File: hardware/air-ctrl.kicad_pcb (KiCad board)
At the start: 2 copper layers, 35 x 35 mm, 71 parts, among them J1 USB_C_Receptacle_USB2.0_16P, J2 SFV24R-2STE1HLF, J3 Conn_ARM_SWD_TagConnect_TC203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, J4 Conn_01x02, Q1 BSS138, SW1 SW_RST, U1 nRF52832-QFxx, U2 BME688, U3 MCP73871-2CC, U4 MCP1700x-330xxTT, Y1 32MHz, Y2 32.768kHz

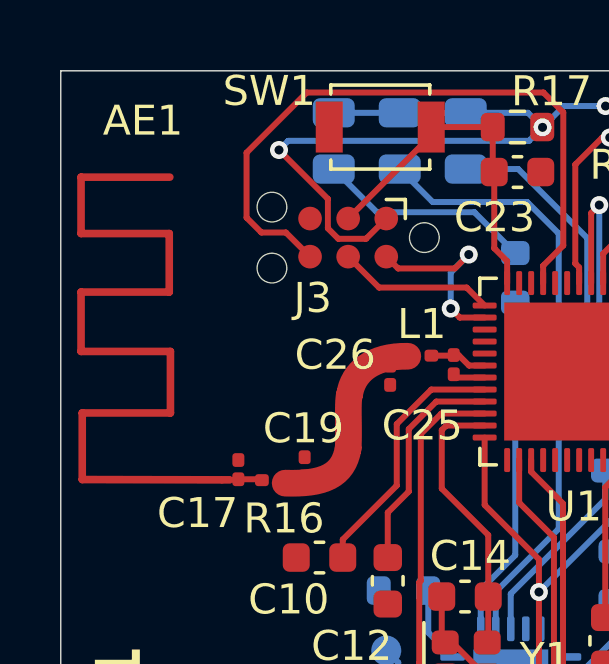
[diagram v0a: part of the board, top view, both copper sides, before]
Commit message: Fixed DRC issues on antenna pad and trace
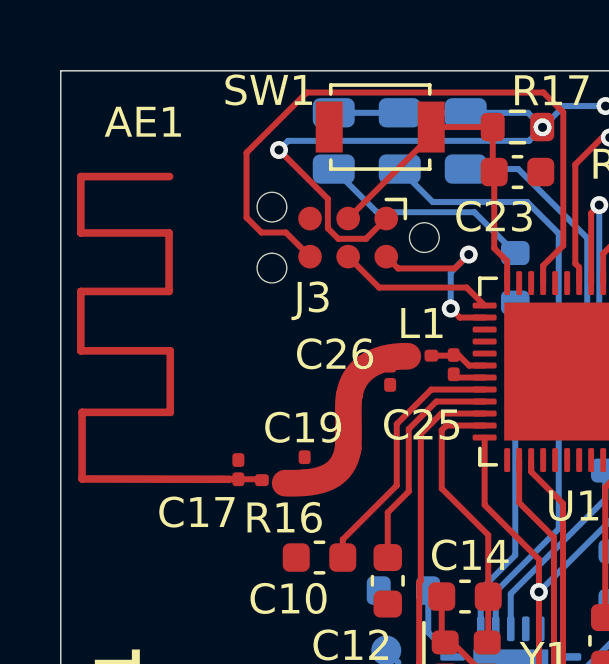
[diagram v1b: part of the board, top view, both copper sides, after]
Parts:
- moved AE1 0.09 mm to (153.7, 48.9)
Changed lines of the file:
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@@
 	(footprint "RF_Antenna:Antenna_BLE"
 		(layer "F.Cu")
-		(at 153.6565 48.81 90)
+		(at 153.71 48.88 90)
 		(property "Reference" "AE1"
 			(at 7.17 -0.9165 0)
@@
 		(net_tie_pad_groups "1")
 		(fp_line
-			(start 5.29 -2.98)
-			(end 5.29 -0.02)
+			(start 5.380104 -3.04)
+			(end 5.380104 -0.08)
 			(stroke
 				(width 0.254)
@@
 		)
 		(fp_line
-			(start 3.41 -2.98)
-			(end 5.29 -2.98)
+			(start 3.500104 -3.04)
+			(end 5.380104 -3.04)
 			(stroke
 				(width 0.254)
@@
 		)
 		(fp_line
-			(start 1.46 -2.98)
-			(end 1.46 -0.04)
+			(start 1.550104 -3.04)
+			(end 1.550104 -0.1)
 			(stroke
 				(width 0.254)
@@
 		)
 		(fp_line
-			(start -0.52 -2.98)
-			(end 1.46 -2.98)
+			(start -0.429896 -3.04)
+			(end 1.550104 -3.04)
 			(stroke
 				(width 0.254)
@@
 		)
 		(fp_line
-			(start -2.57 -2.94)
-			(end -2.57 0)
+			(start -2.479896 -3)
+			(end -2.479896 -0.06)
 			(stroke
 				(width 0.254)
@@
 		)
 		(fp_line
-			(start -4.79 -2.94)
-			(end -2.57 -2.94)
+			(start -4.699896 -3)
+			(end -2.479896 -3)
 			(stroke
 				(width 0.254)
@@
 		)
 		(fp_line
-			(start 3.41 -0.04)
-			(end 3.41 -2.98)
+			(start 3.500104 -0.1)
+			(end 3.500104 -3.04)
 			(stroke
 				(width 0.254)
@@
 		)
 		(fp_line
-			(start 1.46 -0.04)
-			(end 3.41 -0.04)
+			(start 1.550104 -0.1)
+			(end 3.500104 -0.1)
 			(stroke
 				(width 0.254)
@@
 		)
 		(fp_line
-			(start -0.52 0)
-			(end -0.52 -2.98)
+			(start -0.429896 -0.06)
+			(end -0.429896 -3.04)
 			(stroke
 				(width 0.254)
@@
 		)
 		(fp_line
-			(start -2.57 0)
-			(end -0.52 0)
+			(start -2.479896 -0.06)
+			(end -0.429896 -0.06)
 			(stroke
 				(width 0.254)
@@
 		)
 		(fp_line
-			(start -4.8 1.7)
-			(end -4.790104 -2.94)
+			(start -4.709896 1.64)
+			(end -4.7 -3)
 			(stroke
 				(width 0.254)
@@
 		)
 		(pad "1" connect roundrect
-			(at -4.8 1.85 180)
+			(at -4.709896 1.79 180)
 			(size 0.377 0.254)
 			(layers "F.Cu" "F.Mask")
@@
 		)
 		(group ""
-			(members "209a0455-04f6-4b58-b0ae-014dd7f7e8bc" "2509789c-07dd-4dd8-a51f-43c243804211"
-				"26a550a0-0e9e-42ae-ae6a-5513f2a037a7" "2a4eed77-9d9f-4b0f-ba56-ba25d8e712e8"
-				"4f7e4597-fbac-4e23-aed2-afa333fae4f6" "55c94455-214e-4ffb-a6da-015bdf38ccf6"
-				"705c0e73-2bbe-4a66-b21e-bebf5369d946" "994df067-cb94-43e8-8fc0-f8c08f739cad"
-				"d8a0ef51-1bcc-4bfa-a21e-0bc05fa7d346" "e0c5d7c5-d813-4090-9b40-0154119800ae"
-				"e7c0935a-e132-4bfe-911e-57bb95cab03a" "ff8d8c75-0cb4-45cd-b153-e8660f922aba"
+			(members "28919dec-981b-449c-8571-14b3c1193a38" "36499084-ff91-43a0-9559-5762354c162e"
+				"40a73ee6-07f7-4537-9c1d-6c57c1513f92" "5895e3f0-3bd3-41a0-b642-3b390754c57b"
+				"62b5ca1d-d3de-4e46-8a23-bc883b20b2ab" "6c8e7c77-08ca-4a85-ba5d-5a3286ddfb7c"
+				"75b1eca4-620c-4eff-8bdc-2bc21a9c6d79" "8d3f4351-a146-4af2-b67d-fe788fbdf3c5"
+				"afcf701b-003e-42b7-b24e-b941a6066965" "b3a84e2a-ce09-4ddf-ade8-84811e1e0511"
+				"c99fd7f9-daf0-4e98-9e11-d4545e4ea354" "e7c0935a-e132-4bfe-911e-57bb95cab03a"
 			)
 		)
@@
 	)
 	(segment
-		(start 155.5065 53.61)
-		(end 155.9 53.61)
+		(start 155.678274 53.59)
+		(end 155.677999 53.590275)
 		(width 0.2)
 		(layer "F.Cu")
@@
 	)
 	(segment
+		(start 155.92 53.59)
+		(end 155.678274 53.59)
+		(width 0.2)
+		(layer "F.Cu")
+		(net 1)
+	)
+	(segment
 		(start 156.675 53.59)
 		(end 156.705 53.62)
@@
 		(polygon
 			(pts
-				(xy 149.95 39.85) (xy 149.95 54.8) (xy 155.35 54.8) (xy 155.35 39.86)
+				(xy 149.95 39.85) (xy 149.95 54.8) (xy 155.35 54.8) (xy 155.35 53.91) (xy 155.2 53.91) (xy 155.2 53.3)
+				(xy 155.35 53.3) (xy 155.35 39.86)
 			)
 		)
